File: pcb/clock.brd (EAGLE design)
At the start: 140 x 50 mm, 33 parts, among them IC1 STM32F072C8T6, IC3 24C64ST

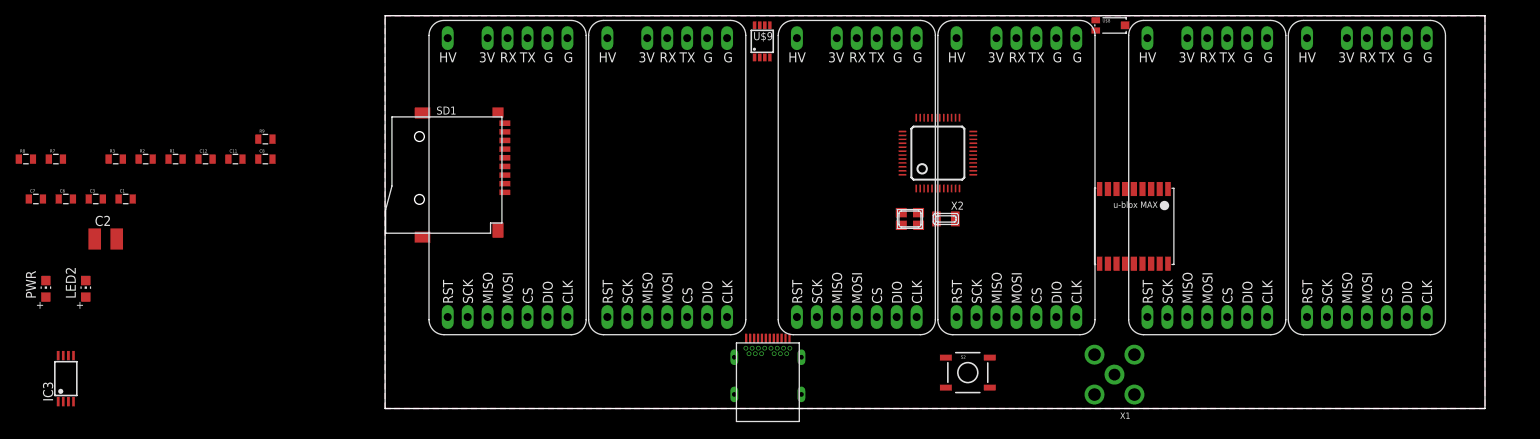
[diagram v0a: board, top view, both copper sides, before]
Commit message: positioned boards
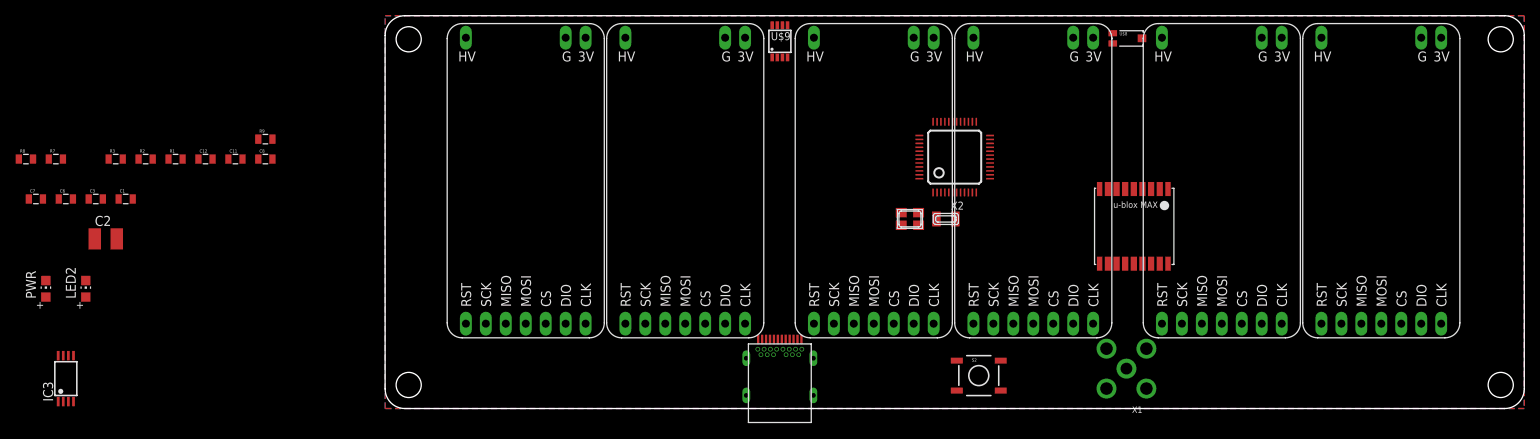
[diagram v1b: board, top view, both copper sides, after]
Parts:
- removed SD1: TF-HOLDER, basicBoard:TF-PULL
- added U$10, U$11, U$12, U$13: M3_MOUNTING_HOLE, a:M3_MOUNTING_HOLE_PACK
- moved U$8 2.72 mm to (94.5, 47.1)
- moved U$1 2.35 mm to (7.90, 9.00)
- moved U$2 2.33 mm to (28.2, 9.00)
- moved U$9 2.24 mm to (50.2, 46.7)
- moved IC1 2.20 mm to (72.5, 32.0)
- moved U$3 2.20 mm to (52.2, 9.00)
- moved U$4 2.18 mm to (72.5, 9.00)
- moved U$5 1.89 mm to (96.5, 9.00)
- moved U$6 1.87 mm to (116.8, 9.00)
- moved X1 1.70 mm to (94.4, 5.08)
- moved CONN1 1.53 mm to (50.2, -1.78)
- moved S2 1.45 mm to (75.6, 4.19)
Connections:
- removed net VDD: SD1.4
- removed net VSS: SD1.6
- net +3V3: now also U$1.3V, U$2.3V, U$3.3V, U$4.3V, U$5.3V, U$6.3V; no longer U$1.VCC, U$2.VCC, U$3.VCC, U$4.VCC, U$5.VCC, U$6.VCC
- net GND: no longer U$1.GND2, U$2.GND2, U$3.GND2, U$4.GND2, U$5.GND2, U$6.GND2
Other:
- board size 140 x 50 mm -> 145 x 50 mm
